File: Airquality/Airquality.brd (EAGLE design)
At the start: 70 x 70 mm, 81 parts, among them IC1 SCD41-D-R2, U1 SGP41-D-R4, U3 BMP581, U4 AP22802AW5-7K-3.3V, U5 AP3602AKTR-G1

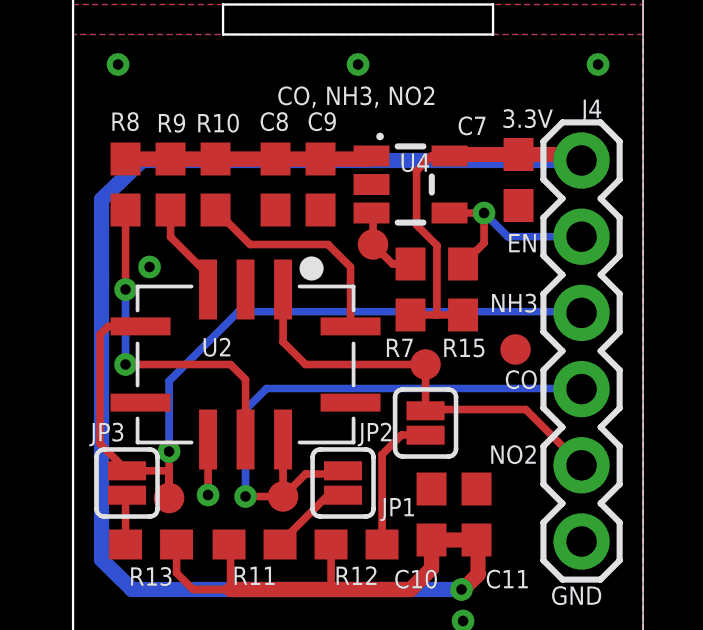
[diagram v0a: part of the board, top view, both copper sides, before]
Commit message: Major Update
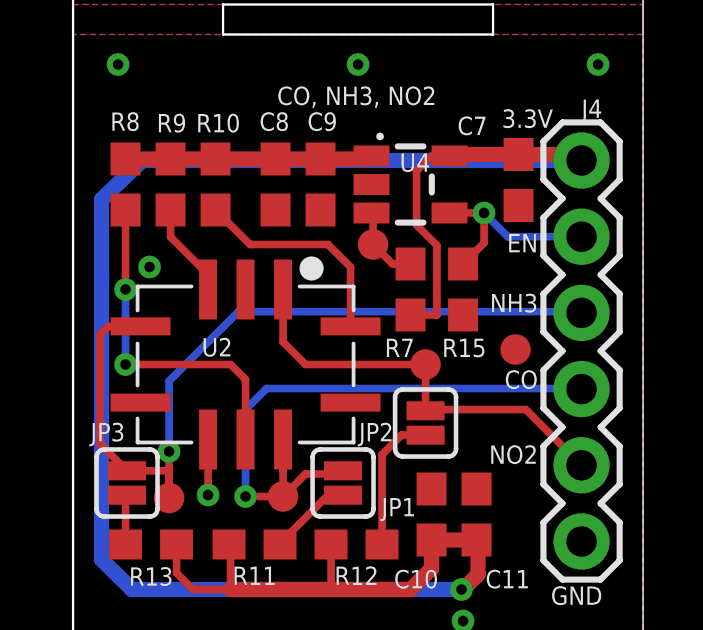
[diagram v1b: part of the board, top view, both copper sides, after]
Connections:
- net 3.3V: no longer R15.1
- net GND: now also R15.1
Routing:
- net 3.3V: track 246.3 -> 245.4 mm
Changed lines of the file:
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@@
 <via x="64" y="16.95" extent="1-16" drill="0.35"/>
 <via x="6.25" y="33.65" extent="1-16" drill="0.35"/>
+<contactref element="R15" pad="1"/>
 <wire x1="60.5" y1="35.5" x2="60.5" y2="38.5" width="0" layer="19" extent="1-1"/>
 </signal>
@@
 <wire x1="6.25" y1="30.65" x2="6.25" y2="32.2" width="0.508" layer="1"/>
 <wire x1="6.25" y1="32.2" x2="5.35" y2="33" width="0.508" layer="16"/>
-<contactref element="R15" pad="1"/>
 <wire x1="62.25" y1="27.15" x2="63.1294" y2="27.15" width="0.254" layer="1"/>
-<wire x1="63.1294" y1="27.15" x2="64" y2="27.15" width="0.254" layer="1"/>
 <wire x1="63.1294" y1="27.15" x2="63.1294" y2="29.4706" width="0.254" layer="1"/>
 <wire x1="63.1294" y1="29.4706" x2="62.45" y2="30.15" width="0.254" layer="1"/>
